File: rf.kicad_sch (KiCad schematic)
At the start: 2 parts, among them U3 RFM95W-868S2

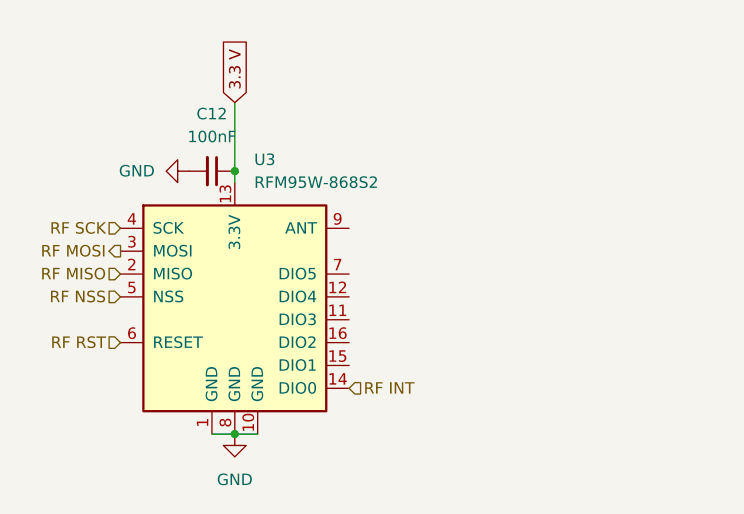
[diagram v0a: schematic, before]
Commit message: Custom RF module and component
Created my own setup for the footprint for the custom RF module
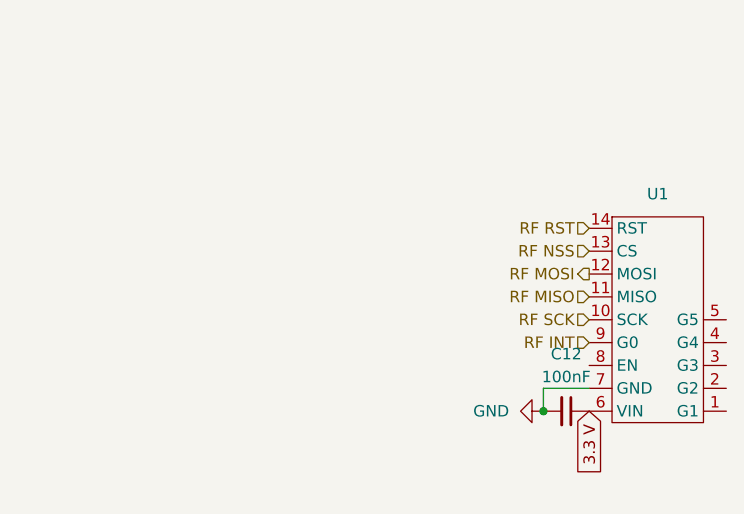
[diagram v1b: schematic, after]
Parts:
- removed U3: RFM95W-868S2, customrf:rf module, symbol RF_Module:RFM95W-868S2
- added U1: (no value), customrf:rf module, symbol X19-Float-Board-eagle-import:rfm95adafruitmodule
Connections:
- net 3.3 V: now also U1.6 (VIN)
- net GND: now also U1.7 (GND)
- net RF INT: now also U1.9 (G0)
- net RF MISO: now also U1.11 (MISO)
- net RF MOSI: now also U1.12 (MOSI)
- net RF NSS: now also U1.13 (CS)
- net RF RST: now also U1.14 (RST)
- net RF SCK: now also U1.10 (SCK)
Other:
- moved on the sheet: C12
